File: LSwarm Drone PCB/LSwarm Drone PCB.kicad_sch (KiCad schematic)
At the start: 27 parts, among them J2 USB_C_Receptacle_USB2.0_16P, SW1 SW_Push_Dual, SW2 SW_Push_Dual, U1 RP2350A, U2 ESP32-C3, U3 LD1117V, U4 W25Q128JVS, Y1 12MHz

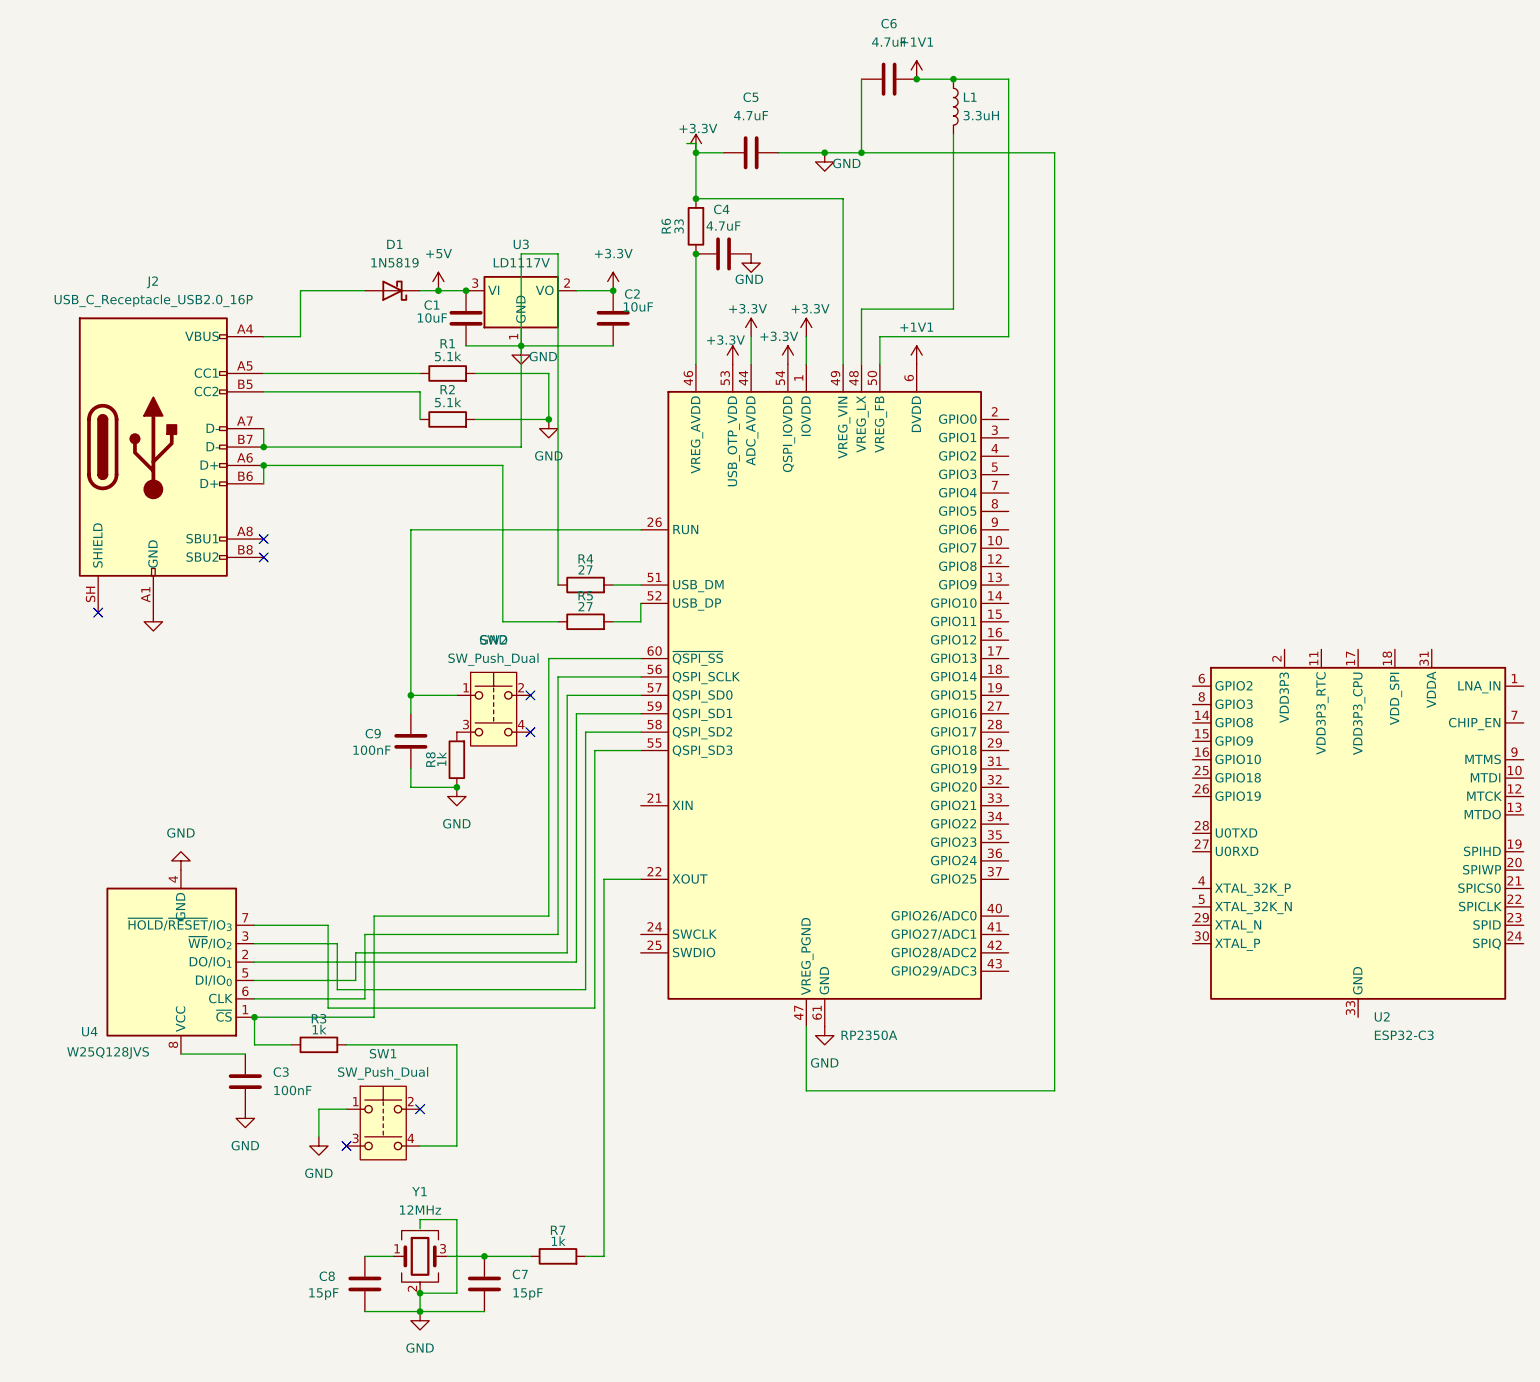
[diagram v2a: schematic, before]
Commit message: sync
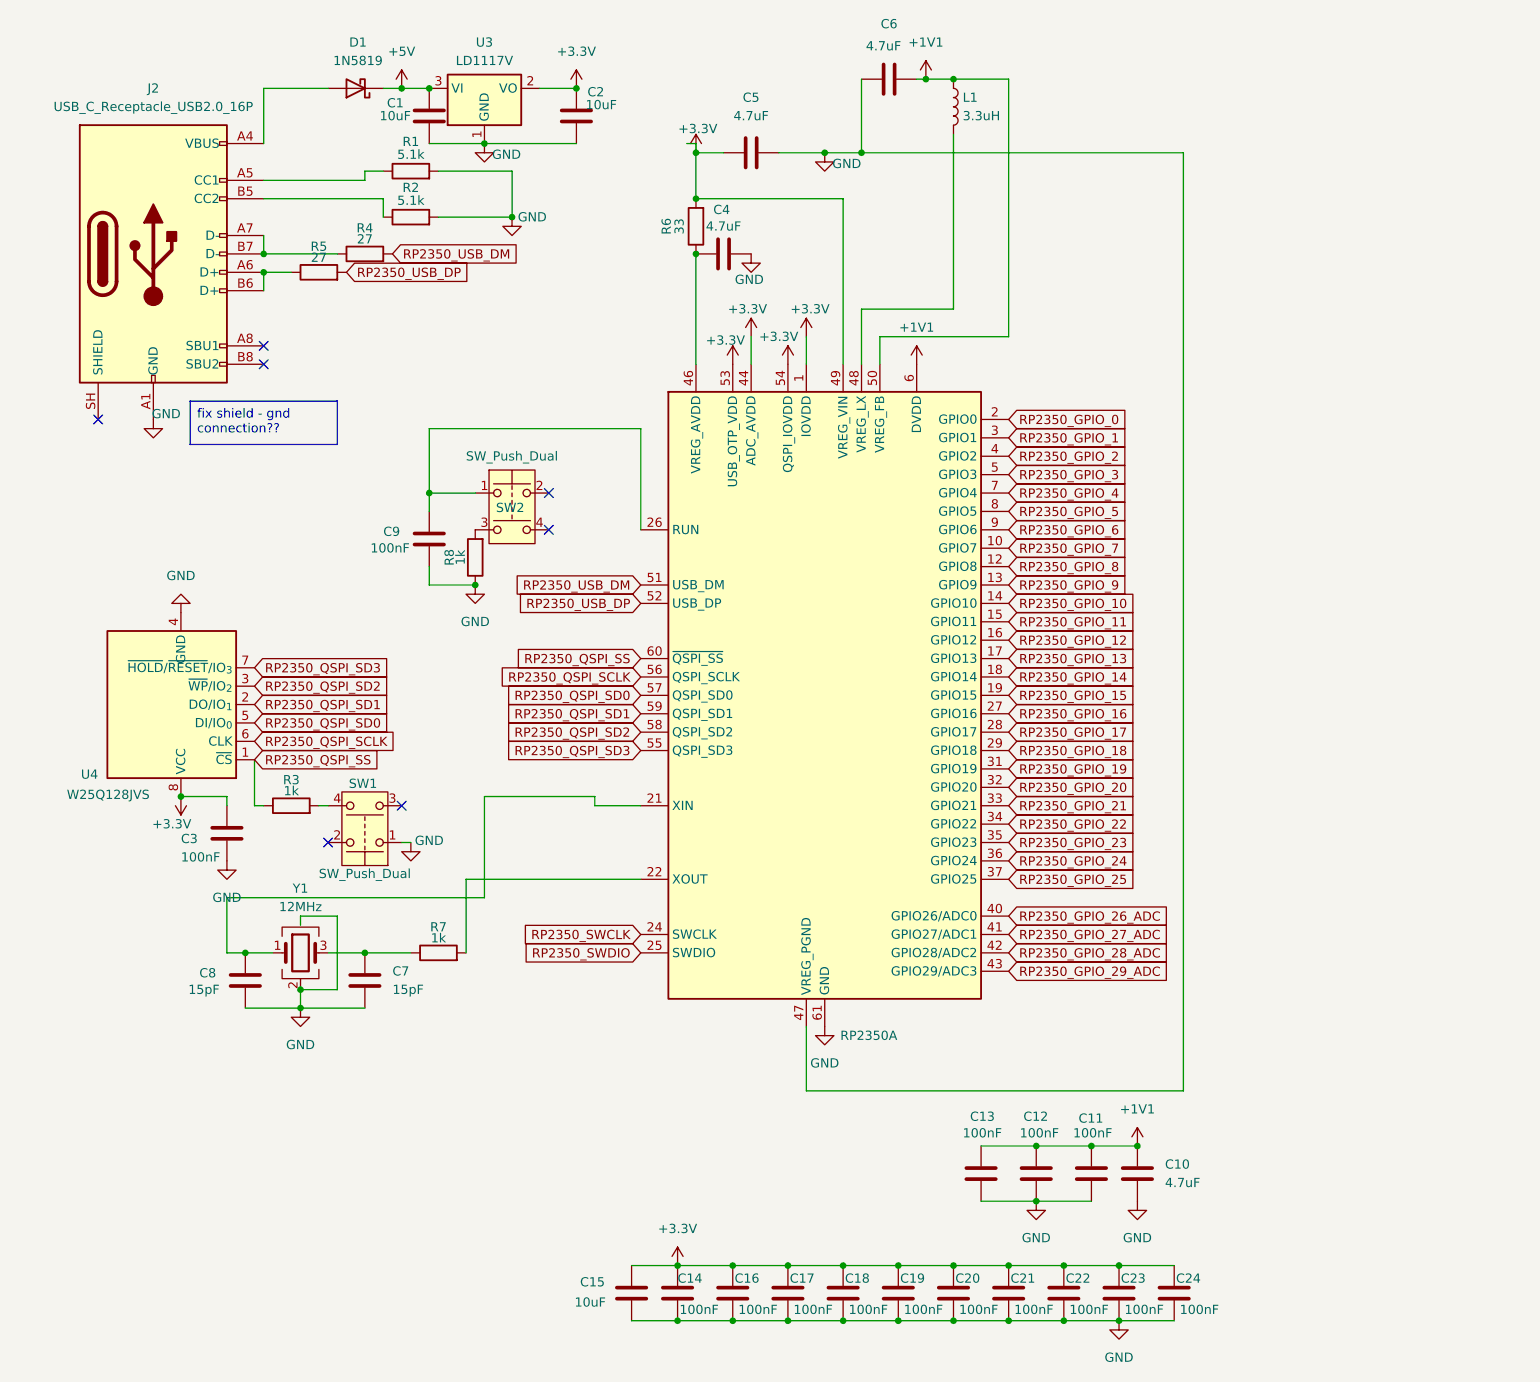
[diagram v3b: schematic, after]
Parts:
- removed U2: ESP32-C3, Package_DFN_QFN:QFN-32-1EP_5x5mm_P0.5mm_EP3.7x3.7mm, symbol MCU_Espressif:ESP32-C3
- added C10: 4.7uF, symbol Device:C
- added C11, C12, C13, C14, C16, C17, C18, C19, C20, C21, C22, C23, C24: 100nF, symbol Device:C
- added C15: 10uF, symbol Device:C
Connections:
- net +1V1: now also C10.1, C11.1, C12.1, C13.1
- net +3.3V: now also C3.1, U4.8 (VCC), C14.1, C15.1, C16.1, C17.1, C18.1, C19.1, C20.1, C21.1, C22.1, C23.1, C24.1
- net GND: now also C10.2, C11.2, C12.2, C13.2, C14.2, C15.2, C16.2, C17.2, C18.2, C19.2, C20.2, C21.2, C22.2, C23.2, C24.2; no longer J2.A7 (D-), J2.B7 (D-), R4.1
- net RP2350_USB_DM: now reaches R4.2, U1.51 (USB_DM)
- net RP2350_QSPI_SS: now reaches R3.1, U1.60 (~{QSPI_SS}), U4.1 (~{CS})
- net at C8.1, Y1.1: now also U1.21 (XIN)
- net RP2350_GPIO_7: now reaches U1.10 (GPIO7)
- net RP2350_GPIO_8: now reaches U1.12 (GPIO8)
- net RP2350_GPIO_9: now reaches U1.13 (GPIO9)
- net RP2350_GPIO_10: now reaches U1.14 (GPIO10)
- net RP2350_GPIO_11: now reaches U1.15 (GPIO11)
- net RP2350_GPIO_12: now reaches U1.16 (GPIO12)
- net RP2350_GPIO_13: now reaches U1.17 (GPIO13)
- net RP2350_GPIO_14: now reaches U1.18 (GPIO14)
- net RP2350_GPIO_15: now reaches U1.19 (GPIO15)
- net RP2350_GPIO_0: now reaches U1.2 (GPIO0)
- net RP2350_SWCLK: now reaches U1.24 (SWCLK)
- net RP2350_SWDIO: now reaches U1.25 (SWDIO)
- net RP2350_GPIO_16: now reaches U1.27 (GPIO16)
- net RP2350_GPIO_17: now reaches U1.28 (GPIO17)
- net RP2350_GPIO_18: now reaches U1.29 (GPIO18)
- net RP2350_GPIO_1: now reaches U1.3 (GPIO1)
- net RP2350_GPIO_19: now reaches U1.31 (GPIO19)
- net RP2350_GPIO_20: now reaches U1.32 (GPIO20)
- net RP2350_GPIO_21: now reaches U1.33 (GPIO21)
- net RP2350_GPIO_22: now reaches U1.34 (GPIO22)
- net RP2350_GPIO_23: now reaches U1.35 (GPIO23)
- net RP2350_GPIO_24: now reaches U1.36 (GPIO24)
- net RP2350_GPIO_25: now reaches U1.37 (GPIO25)
- net RP2350_GPIO_2: now reaches U1.4 (GPIO2)
- net RP2350_GPIO_26_ADC: now reaches U1.40 (GPIO26/ADC0)
- net RP2350_GPIO_27_ADC: now reaches U1.41 (GPIO27/ADC1)
- net RP2350_GPIO_28_ADC: now reaches U1.42 (GPIO28/ADC2)
- net RP2350_GPIO_29_ADC: now reaches U1.43 (GPIO29/ADC3)
- net RP2350_GPIO_3: now reaches U1.5 (GPIO3)
- net RP2350_USB_DP: now reaches R5.2, U1.52 (USB_DP)
- net RP2350_QSPI_SD3: now reaches U1.55 (QSPI_SD3), U4.7 (~{HOLD}/~{RESET}/IO_{3})
- net RP2350_QSPI_SCLK: now reaches U1.56 (QSPI_SCLK), U4.6 (CLK)
- net RP2350_QSPI_SD0: now reaches U1.57 (QSPI_SD0), U4.5 (DI/IO_{0})
- net RP2350_QSPI_SD2: now reaches U1.58 (QSPI_SD2), U4.3 (~{WP}/IO_{2})
- net RP2350_QSPI_SD1: now reaches U1.59 (QSPI_SD1), U4.2 (DO/IO_{1})
- net RP2350_GPIO_4: now reaches U1.7 (GPIO4)
- net RP2350_GPIO_5: now reaches U1.8 (GPIO5)
- net RP2350_GPIO_6: now reaches U1.9 (GPIO6)
- new net: J2.A7 (D-), J2.B7 (D-), R4.1
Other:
- moved on the sheet: C1, C2, C3, C7, C8, C9, D1, J2, R1, R2, R3, R4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

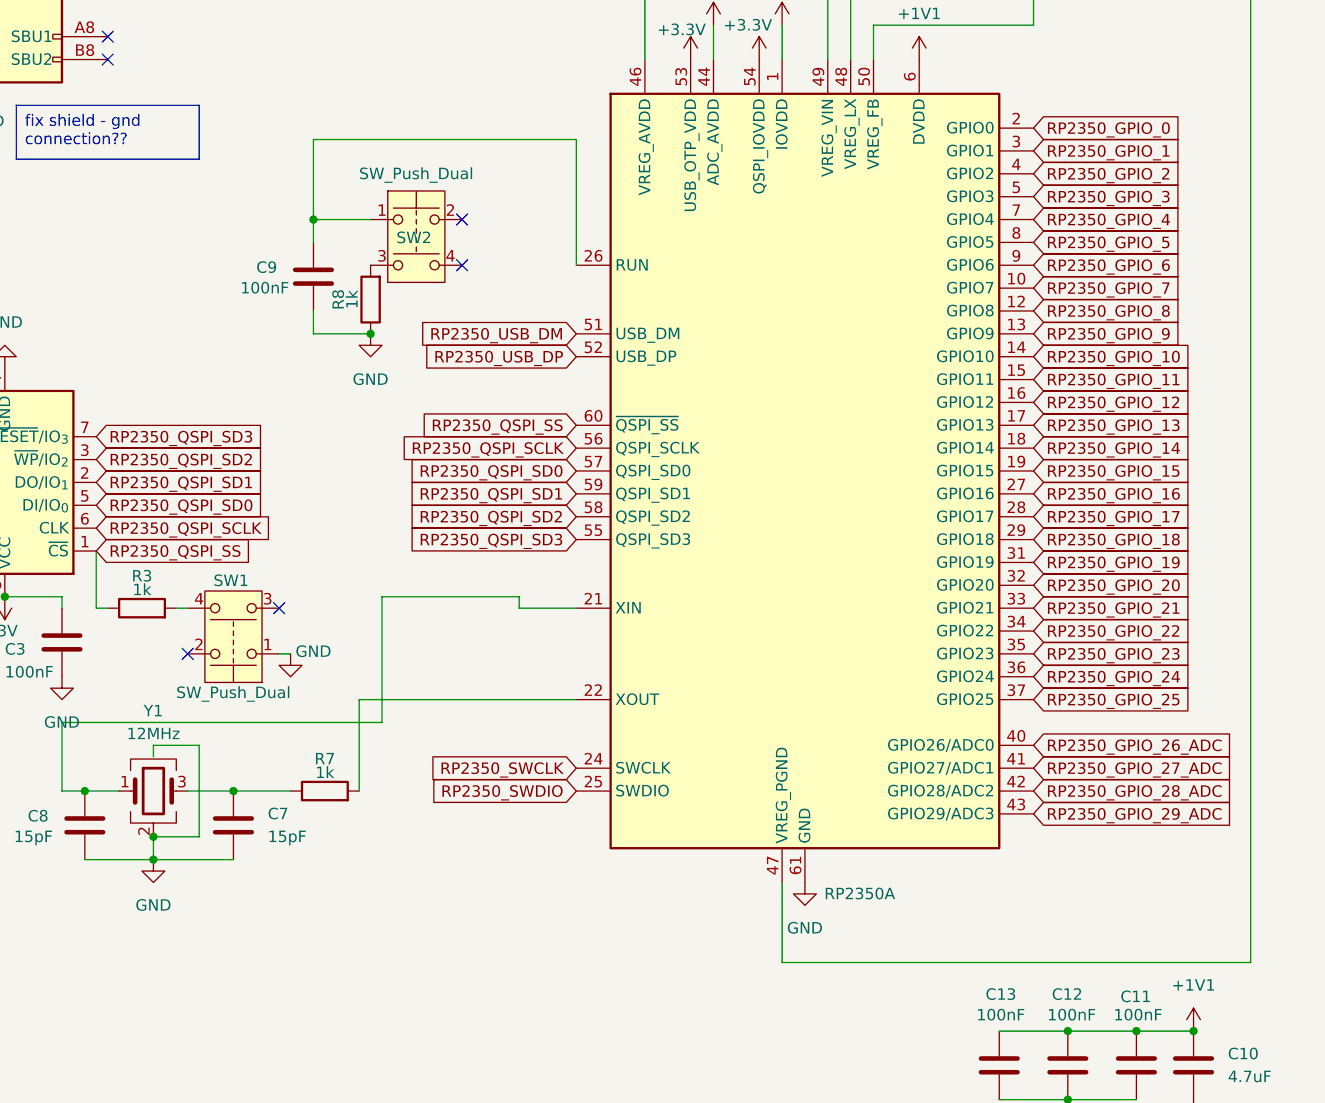
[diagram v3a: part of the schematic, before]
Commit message: sync
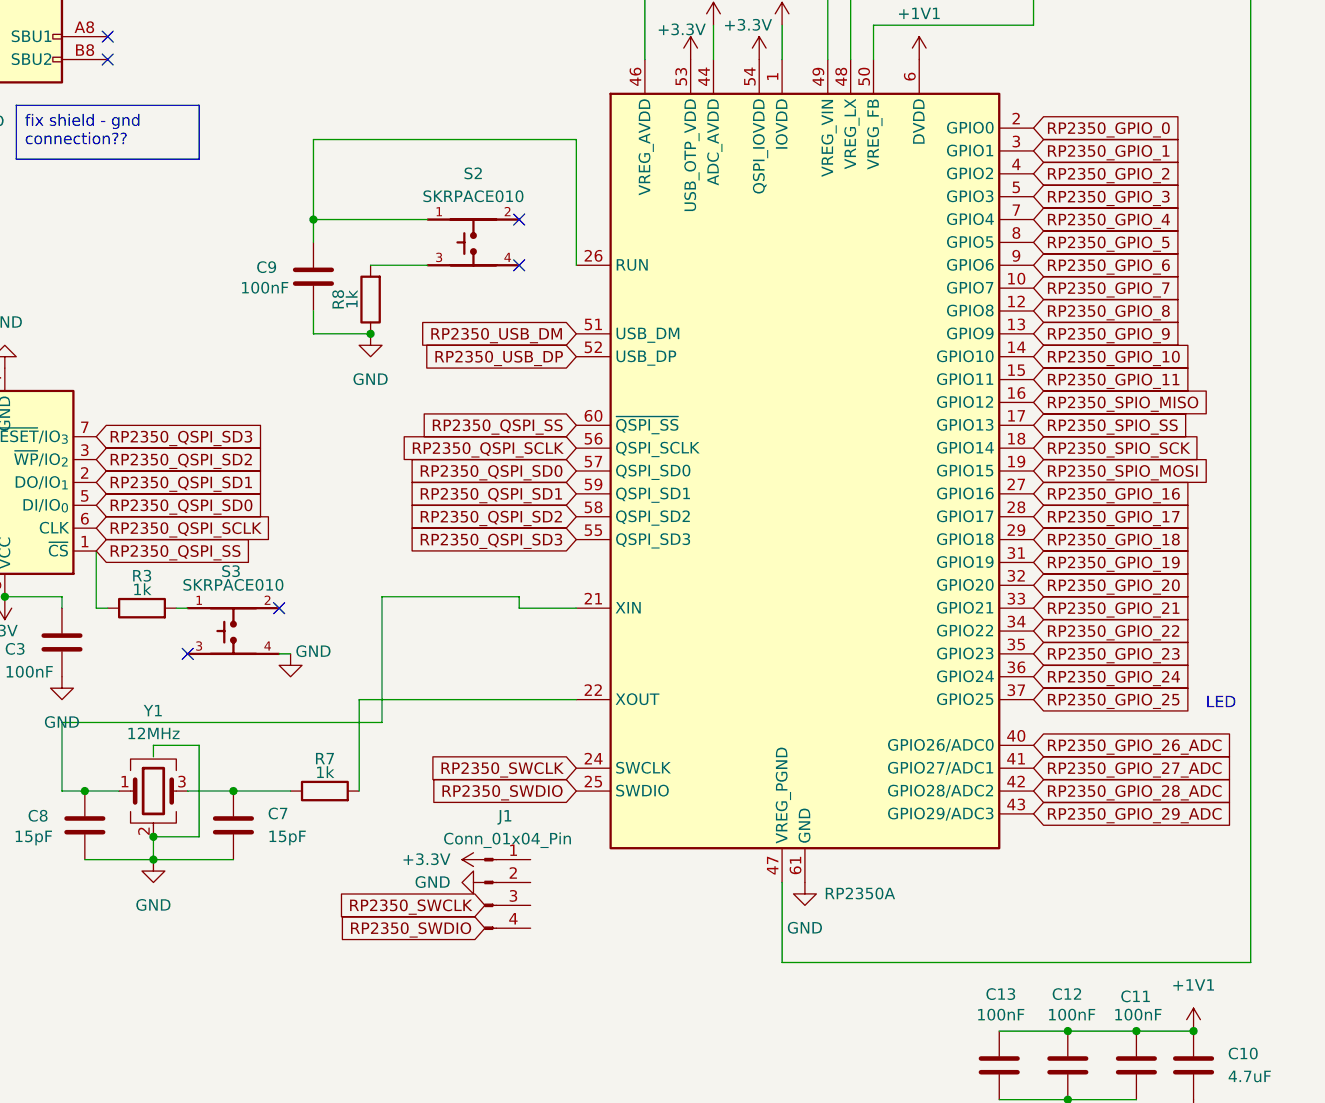
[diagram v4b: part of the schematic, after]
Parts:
- removed SW1, SW2: SW_Push_Dual, symbol Switch:SW_Push_Dual
- added J1: Conn_01x04_Pin, symbol Connector:Conn_01x04_Pin
- added S2, S3: SKRPACE010, SKRPACE010:SW_SKRPACE010, symbol SKRPACE010:SKRPACE010
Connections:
- net GND: now also S3.4
- net at C9.1, U1.26 (RUN): now also S2.1
- net at R8.2: now also S2.3
- net at R3.2: now also S3.1
- net RP2350_GPIO_12 renamed RP2350_SPIO_MISO
- net RP2350_GPIO_13 renamed RP2350_SPIO_SS
- net RP2350_GPIO_14 renamed RP2350_SPIO_SCK
- net RP2350_GPIO_15 renamed RP2350_SPIO_MOSI
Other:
- note added: "LED"
